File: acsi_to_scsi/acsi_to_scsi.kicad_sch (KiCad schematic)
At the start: 14 parts, among them J1 Conn_02x25_Odd_Even, U1 74ALS573, U10 74LS02, U11 74ALS74, U2 74ALS540, U3 74ALS540, U4 74LS01, U5 74ALS74, U6 74ALS08, U7 74ALS85, U8 74LS04, U9 74LS08

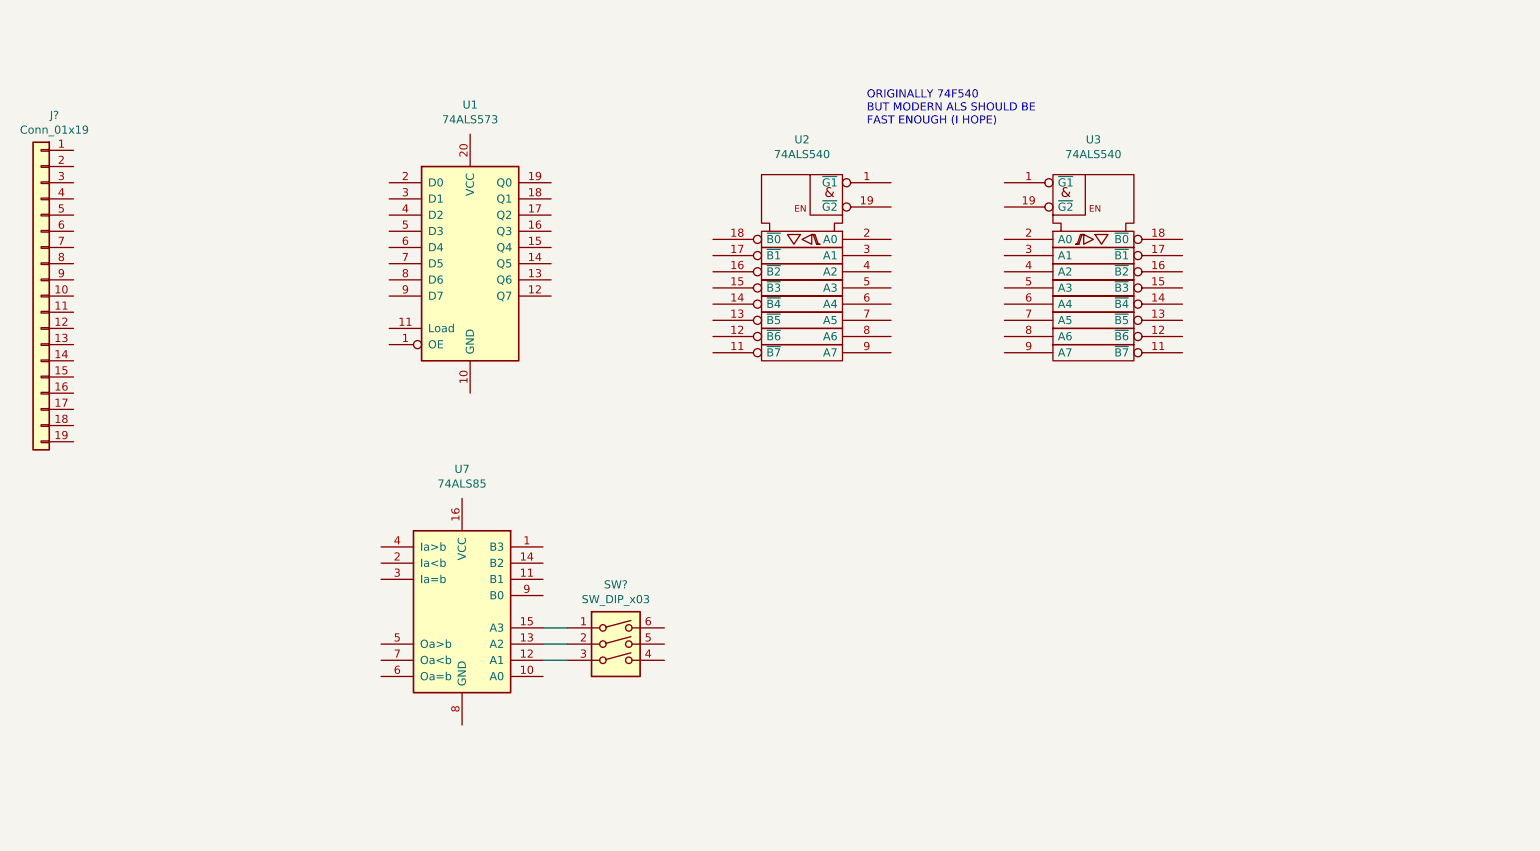
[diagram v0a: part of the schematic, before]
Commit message: a
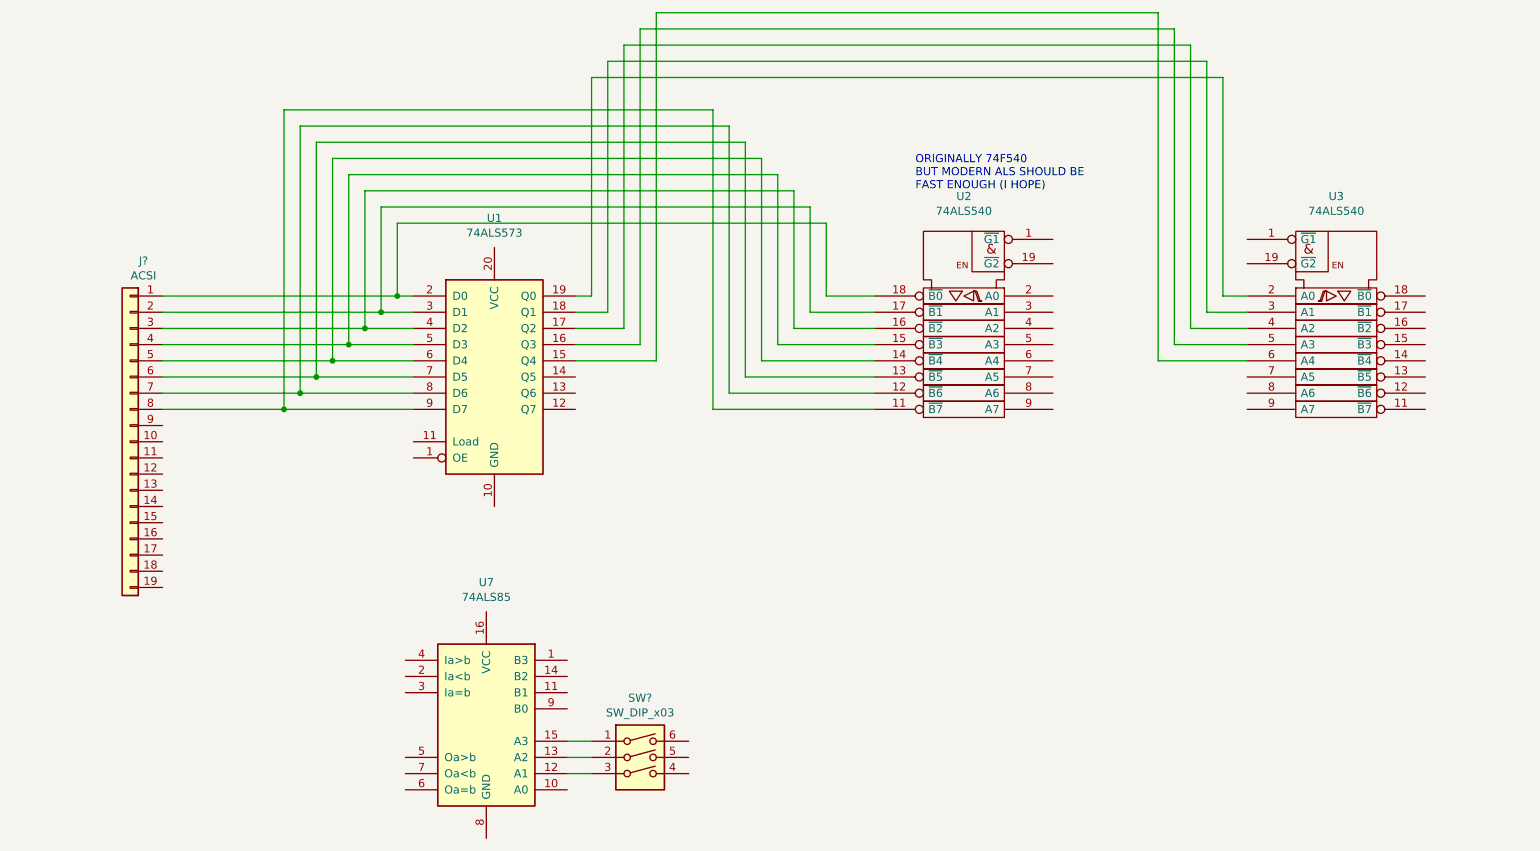
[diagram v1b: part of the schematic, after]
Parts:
- J?: value Conn_01x19 -> ACSI
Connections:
- net at U1.15 (Q4): now also U3.6 (A4)
- net at U1.16 (Q3): now also U3.5 (A3)
- net at U1.17 (Q2): now also U3.4 (A2)
- net at U1.18 (Q1): now also U3.3 (A1)
- net at U1.19 (Q0): now also U3.2 (A0)
- net at U1.2 (D0): now also J?.1 (Pin_1), U2.18 (~B0)
- net at U1.3 (D1): now also J?.2 (Pin_2), U2.17 (~B1)
- net at U1.4 (D2): now also J?.3 (Pin_3), U2.16 (~B2)
- net at U1.5 (D3): now also J?.4 (Pin_4), U2.15 (~B3)
- net at U1.6 (D4): now also J?.5 (Pin_5), U2.14 (~B4)
- net at U1.7 (D5): now also J?.6 (Pin_6), U2.13 (~B5)
- net at U1.8 (D6): now also J?.7 (Pin_7), U2.12 (~B6)
- net at U1.9 (D7): now also J?.8 (Pin_8), U2.11 (~B7)
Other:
- moved on the sheet: J?, SW?, U1, U2, U3, U7

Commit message: a
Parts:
- J1: value Conn_02x25_Odd_Even -> SCSI
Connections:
- net GND: now also J1.1 (Pin_1), J1.11 (Pin_11), J1.13 (Pin_13), J1.15 (Pin_15), J1.17 (Pin_17), J1.19 (Pin_19), J1.21 (Pin_21), J1.23 (Pin_23), J1.27 (Pin_27), J1.29 (Pin_29), J1.3 (Pin_3), J1.31 (Pin_31), J1.33 (Pin_33), J1.35 (Pin_35), J1.37 (Pin_37), J1.39 (Pin_39), J1.41 (Pin_41), J1.43 (Pin_43), J1.45 (Pin_45), J1.47 (Pin_47), J1.49 (Pin_49), J1.5 (Pin_5), J1.7 (Pin_7), J1.9 (Pin_9)
- net at U3.7 (A5): now also U6.3
- net at U3.8 (A6): now also U6.11
- net at U3.9 (A7): now also U6.6
- net at U6.2: now also U6.10, U6.13, U6.5
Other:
- moved on the sheet: J1, U10A, U10B, U10C, U10D, U10E, U11A, U11B, U11C, U4A, U4B, U4C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

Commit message: a
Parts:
- added U?: 74LS280, symbol 74xx:74LS280
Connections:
- net GND: now also U?.4 (I), U?.7 (GND)
- net at U1.12 (Q7): now also U7.11 (B1)
- net at U1.13 (Q6): now also U7.14 (B2)
- net at U1.14 (Q5): now also U7.1 (B3)
- net D0: now reaches J?.1 (Pin_1), U1.2 (D0), U2.18 (~B0)
- net D1: now reaches J?.2 (Pin_2), U1.3 (D1), U2.17 (~B1)
- net D2: now reaches J?.3 (Pin_3), U1.4 (D2), U2.16 (~B2)
- net D3: now reaches J?.4 (Pin_4), U1.5 (D3), U2.15 (~B3)
- net D4: now reaches J?.5 (Pin_5), U1.6 (D4), U2.14 (~B4)
- net D5: now reaches J?.6 (Pin_6), U1.7 (D5), U2.13 (~B5)
- net D6: now reaches J?.7 (Pin_7), U1.8 (D6), U2.12 (~B6)
- net D7: now reaches J?.8 (Pin_8), U1.9 (D7), U2.11 (~B7)
- net at U3.11 (~B7): now also J1.16 (Pin_16), U?.2 (H)
- net at U3.12 (~B6): now also J1.14 (Pin_14), U?.1 (G)
- net at U3.13 (~B5): now also J1.12 (Pin_12), U?.13 (F)
- net at U3.14 (~B4): now also J1.10 (Pin_10), U?.12 (E)
- net at U3.15 (~B3): now also J1.8 (Pin_8), U?.11 (D)
- net at U3.16 (~B2): now also J1.6 (Pin_6), U?.10 (C)
- net at U3.17 (~B1): now also J1.4 (Pin_4), U?.9 (B)
- net at U3.18 (~B0): now also J1.2 (Pin_2), U?.8 (A)
- net at J1.18 (Pin_18): now also U?.6 (Odd)
- no-connect marks 0 -> 1
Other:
- note added: "U4C on orig"
- moved on the sheet: J1, J?, SW?, U1, U10A, U10B, U10C, U10D, U10E, U11A, U11B, U11C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
